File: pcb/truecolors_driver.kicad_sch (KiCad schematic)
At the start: 28 parts, among them CN1 1.0-3PWT, CN2 47053-1000, Q4 BSS138, SW1 TS-1088-AR02016, U1 AP63205WU-7, U2 CH224A, U3 ESP32-S3-WROOM-1(N8R8), U4 AMS1117-3.3

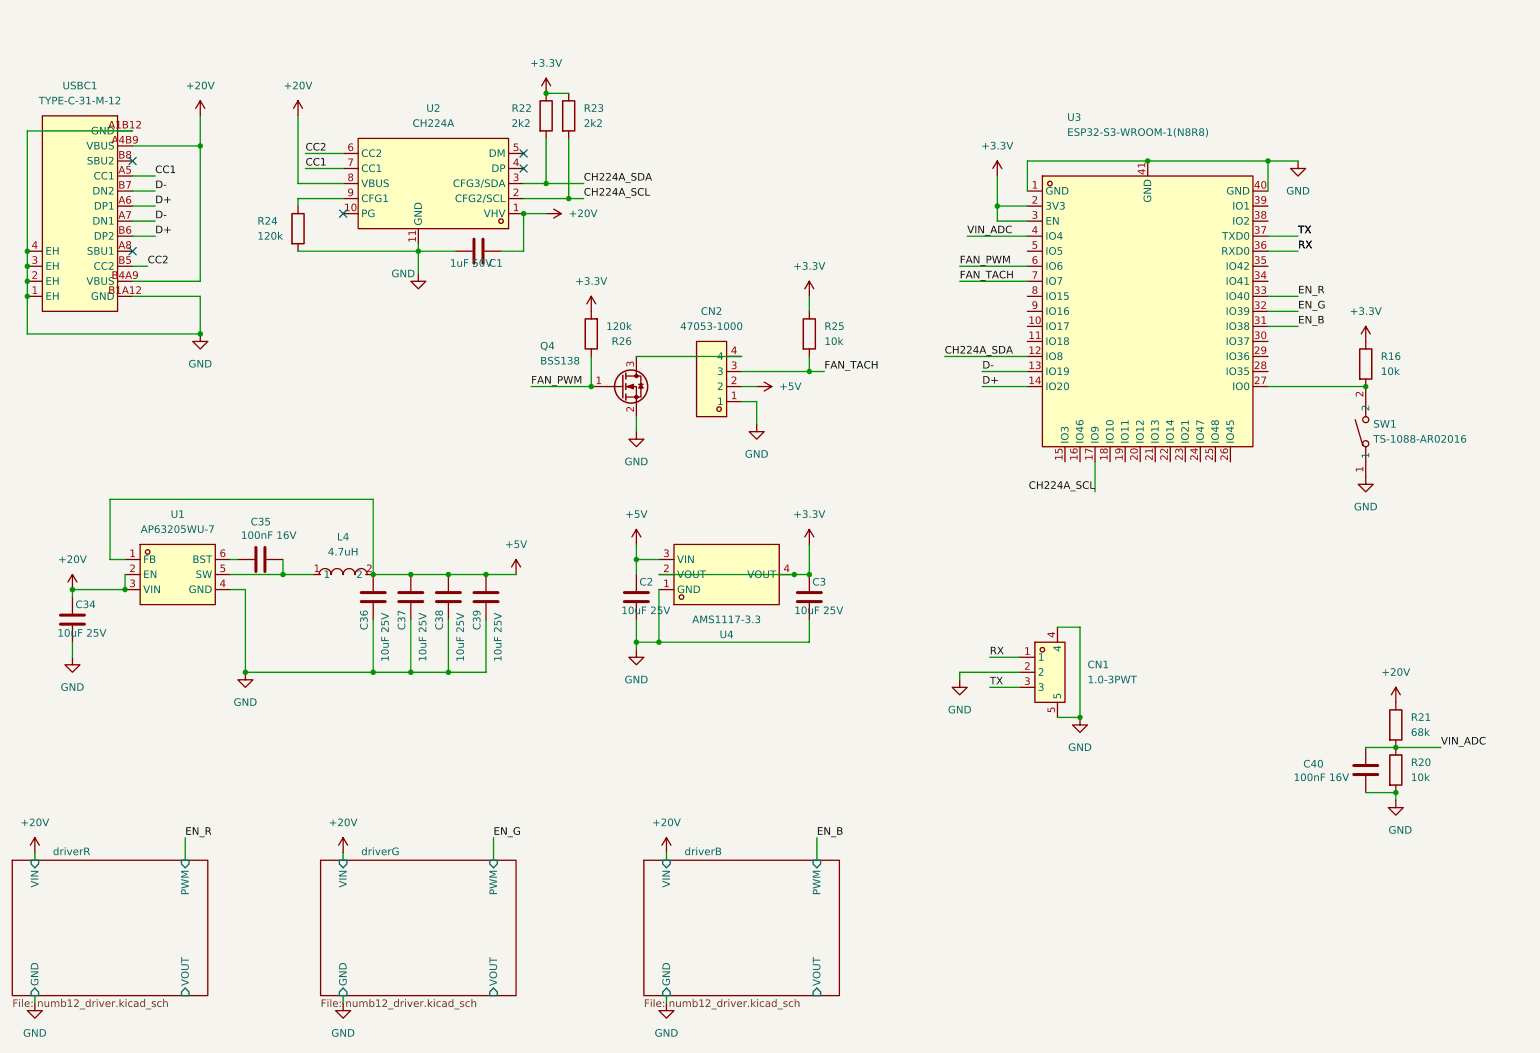
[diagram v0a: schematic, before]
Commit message: add mic, add ntc, fix all drc errors
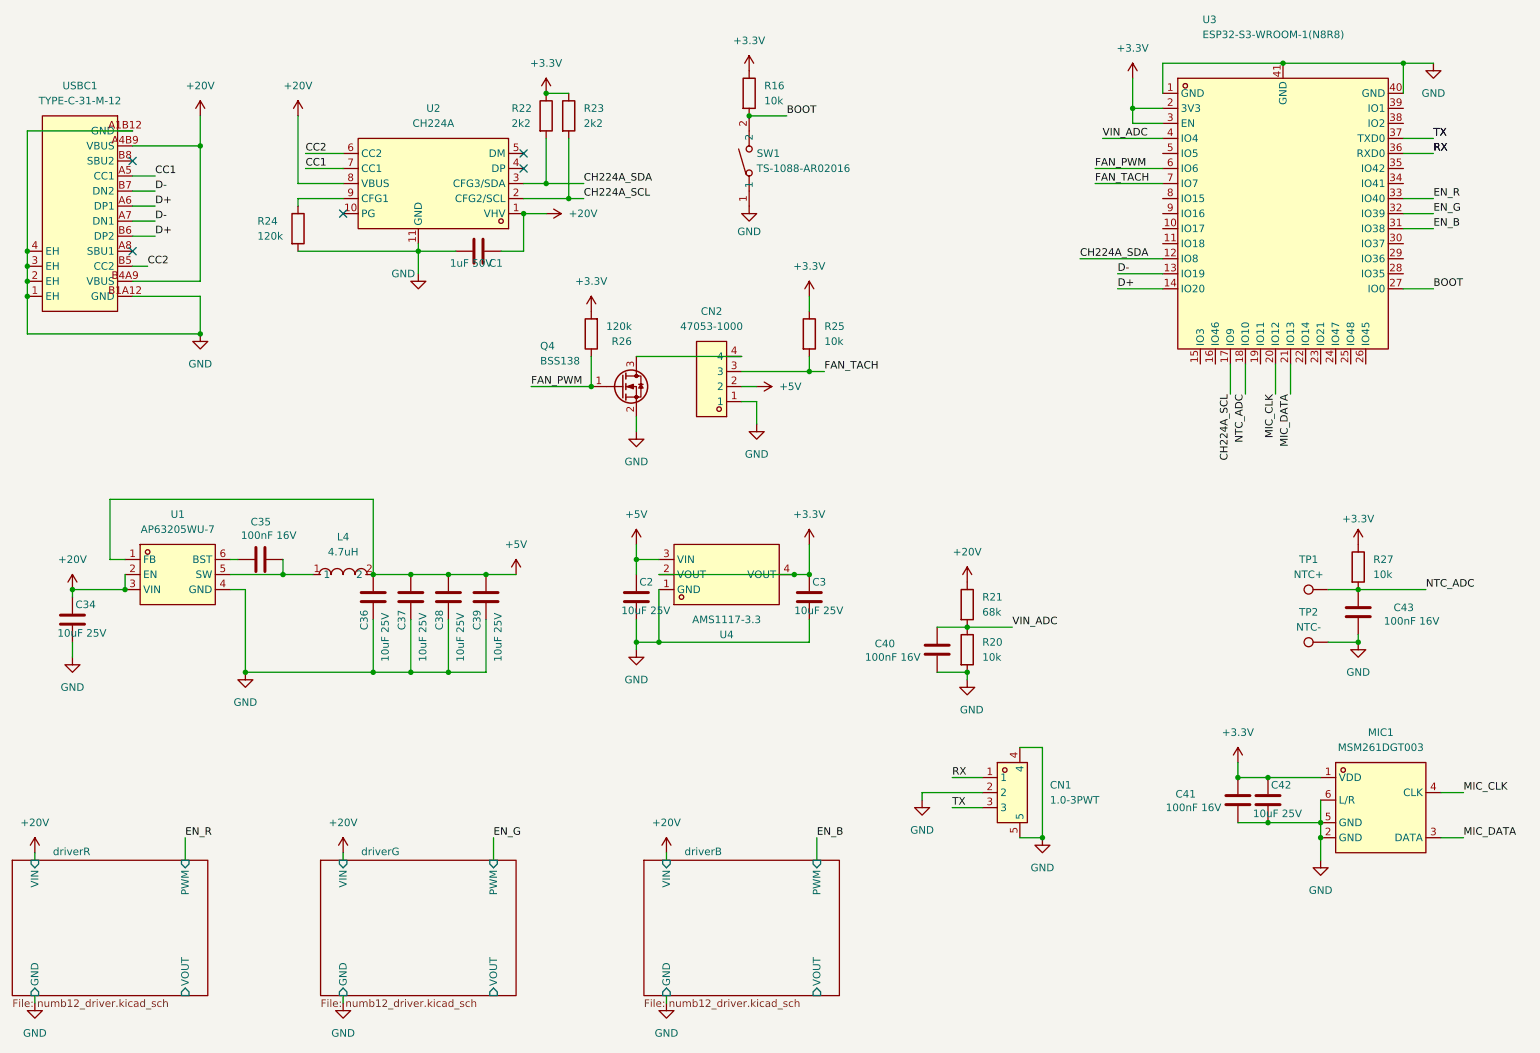
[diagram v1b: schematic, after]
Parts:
- added C41, C43: 100nF 16V, Capacitor_SMD:C_0603_1608Metric, symbol Device:C
- added C42: 10uF 25V, Capacitor_SMD:C_0603_1608Metric, symbol Device:C
- added MIC1: MSM261DGT003, EasyEDA:MIC-SMD_6P-L4.0-W2.0_LMD4020T261-OC3, symbol EasyEDA:MSM261DGT003
- added R27: 10k, Resistor_SMD:R_0603_1608Metric, symbol Device:R
- added TP1: NTC+, TestPoint:TestPoint_Keystone_5019_Miniature, symbol Connector:TestPoint
- added TP2: NTC-, TestPoint:TestPoint_Keystone_5019_Miniature, symbol Connector:TestPoint
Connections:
- net +3.3V: now also C41.2, C42.1, MIC1.1 (VDD), R27.1
- net GND: now also C41.1, C42.2, C43.1, MIC1.2 (GND), MIC1.5 (GND), MIC1.6 (L/R), TP2.1
- net BOOT: now reaches R16.2, SW1.2, U3.27 (IO0)
- net NTC_ADC: now reaches U3.18 (IO10)
- net NTC_ADC: now also C43.2, R27.2, TP1.1
- net MIC_CLK: now reaches U3.20 (IO12)
- net MIC_CLK: now also MIC1.4 (CLK)
- net MIC_DATA: now reaches U3.21 (IO13)
- net MIC_DATA: now also MIC1.3 (DATA)
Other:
- moved on the sheet: C40, CN1, R16, R20, R21, SW1, U3
